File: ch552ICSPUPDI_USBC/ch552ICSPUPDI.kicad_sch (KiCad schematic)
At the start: 18 parts, among them J1 USB_B_Micro, J2 PWR, J3 icsp, J4 UPDI, SW1 SW_SPST, U1 CH552G, U2 AMS1117-3.3

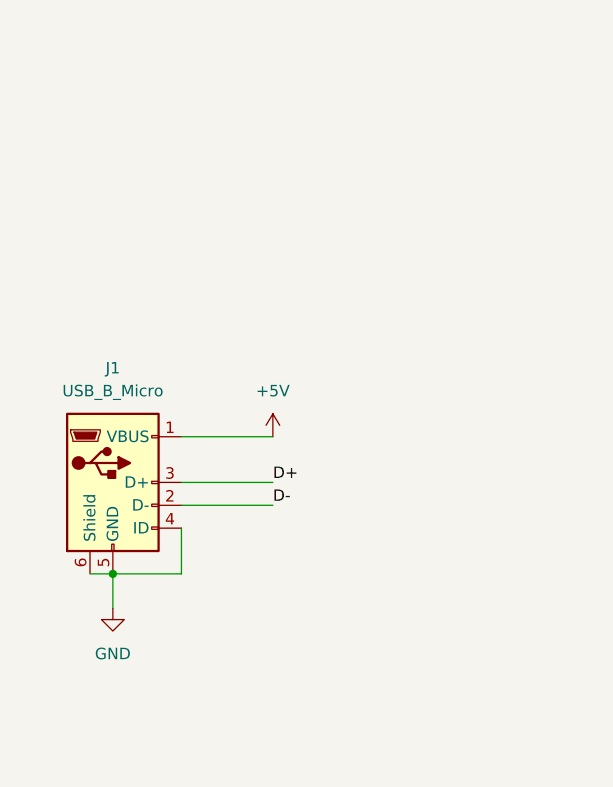
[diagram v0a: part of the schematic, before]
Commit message: update
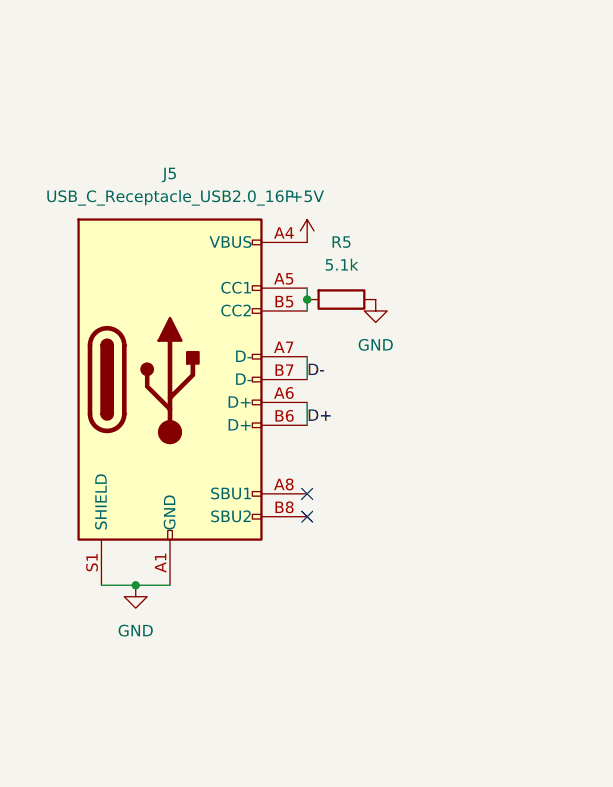
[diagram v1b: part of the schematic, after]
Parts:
- removed J1: USB_B_Micro, Connector_USB:USB_Micro-B_Molex_47346-0001, symbol Connector:USB_B_Micro
- added J5: USB_C_Receptacle_USB2.0_16P, Connector_USB:USB_C_Receptacle_GCT_USB4105-xx-A_16P_TopMnt_Horizontal, symbol Connector:USB_C_Receptacle_USB2.0_16P
- added R5: 5.1k, Resistor_SMD:R_0402_1005Metric_Pad0.72x0.64mm_HandSolder, symbol Device:R
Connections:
- net +5V: now also J5.A4 (VBUS), J5.A9 (VBUS), J5.B4 (VBUS), J5.B9 (VBUS)
- net D+: now also J5.A6 (D+), J5.B6 (D+)
- net D-: now also J5.A7 (D-), J5.B7 (D-)
- net GND: now also J5.A1 (GND), J5.A12 (GND), J5.B1 (GND), J5.B12 (GND), J5.S1 (SHIELD), R5.1
- new net: J5.A5 (CC1), J5.B5 (CC2), R5.2
- no-connect marks 4 -> 6
